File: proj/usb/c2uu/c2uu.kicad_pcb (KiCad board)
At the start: 2 copper layers, 14 x 12 mm, 15 parts, among them J1 USB_C_Receptacle_USB2.0_16P, P1 USB_C_Plug, U1 CH340E, U2 TS5A23159DGS

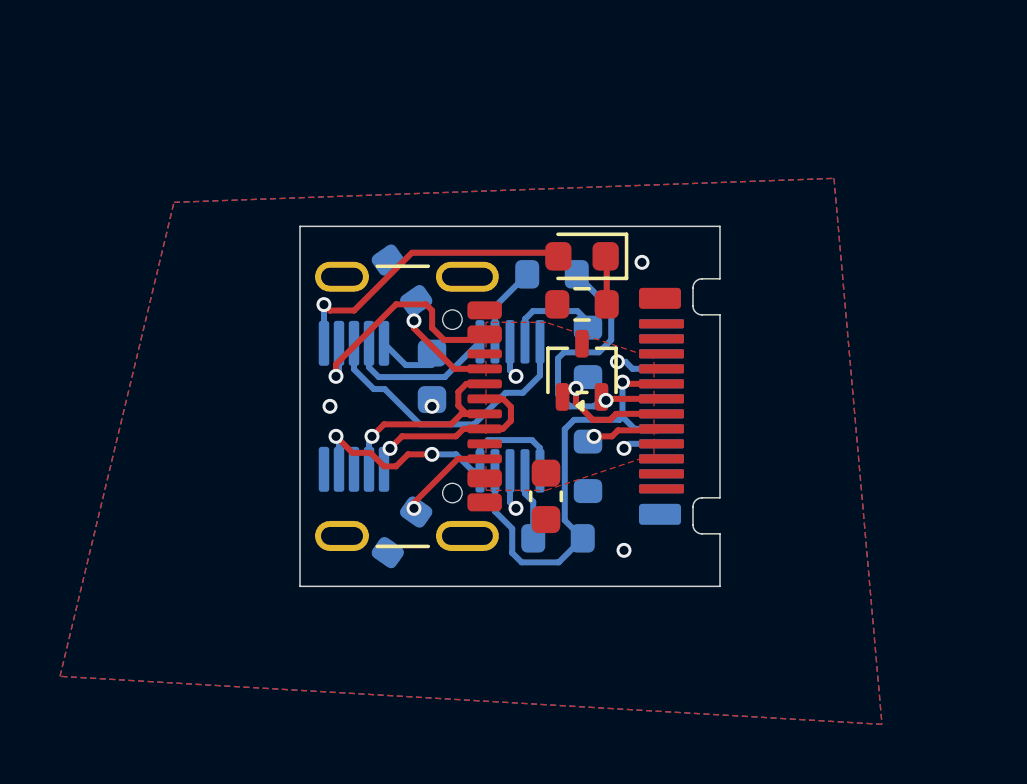
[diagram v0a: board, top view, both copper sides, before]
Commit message: -
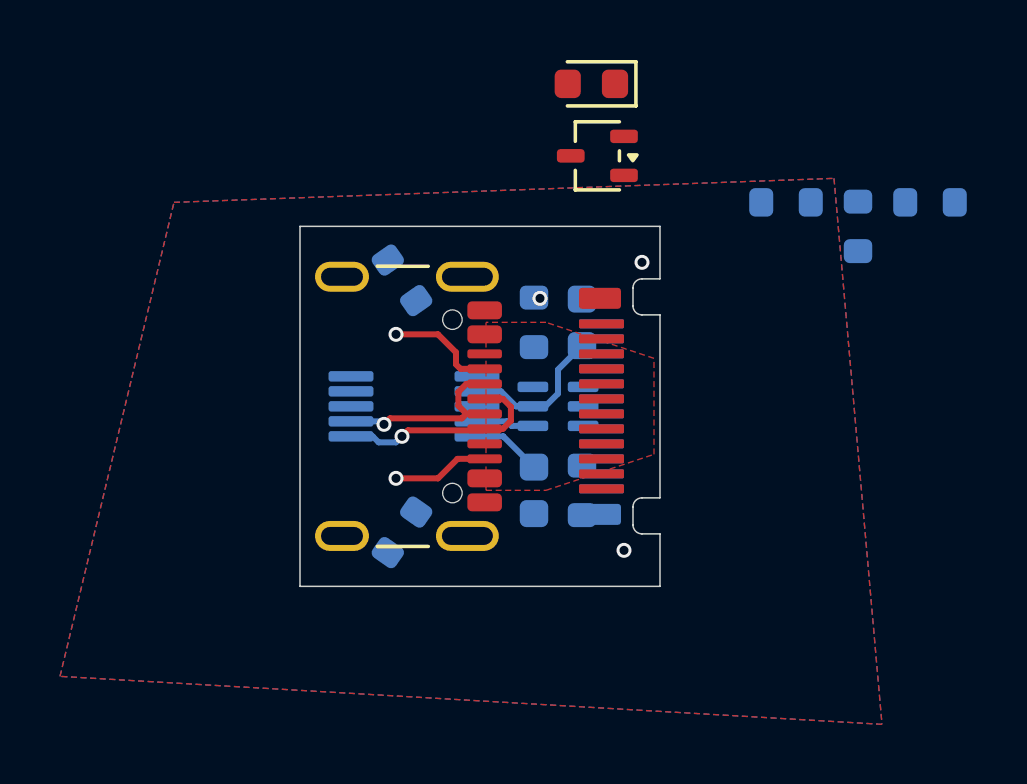
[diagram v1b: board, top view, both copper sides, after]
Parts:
- C1, P1, R7: moved to B.Cu
- U2: value TS5A23159DGS -> 74LVC1G3157; footprint Package_SO:TSSOP-10_3x3mm_P0.5mm -> Package_TO_SOT_SMD:SOT-363_SC-70-6
- moved R5 16.7 mm to (112.0, 93.2)
- moved R4 9.93 mm to (109.6, 94.0)
- moved R6 8.16 mm to (107.2, 93.2)
- moved D2 7.17 mm to (100.9, 91.7), turned to 180 degrees
- moved C1 5.92 mm to (100.4, 97.2), turned to 90 degrees
- moved D1 5.76 mm to (100.7, 89.2)
- moved C2 5.10 mm to (98.8, 102.8)
- moved P1 2.00 mm to (102.1, 100.0), turned to -90 degrees
- moved U1 2.00 mm to (94.8, 100.0), turned to 0 degrees
- moved R7 1.71 mm to (98.8, 97.2), turned to 90 degrees
- moved U2 1.60 mm to (99.6, 100.0), turned to 180 degrees
- moved R3 0.82 mm to (100.4, 102.8)
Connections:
- D1 pad 1: Net-(D1-K) -> GND
- D1 pad 2: TNOW -> Net-(D1-A)
- R4 pad 1: Net-(R4-Pad1) -> TXD
- R5 pad 1: Net-(R5-Pad1) -> TXD
- R7 pad 1: Net-(D1-K) -> TNOW
- R7 pad 2: GND -> Net-(D1-A)
- U2 pad 1: ~{RTS} -> UPDI
- U2 pad 2: Net-(R5-Pad1) -> GND
- U2 pad 3: GND -> Net-(R6-Pad1)
- U2 pad 4: UPDI -> RXD
- U2 pad 5: ~{RTS} -> VBUS
- U2 pad 6: RXD -> ~{RTS}
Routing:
- net UPDI: track 15.5 -> 0.00 mm, vias 1 -> 0
- net ~{RTS}: track 10.5 -> 0.00 mm, vias 2 -> 0
- net TNOW: track 10.0 -> 0.00 mm, vias 1 -> 0
- net UART_IN: track 9.68 -> 0.00 mm, vias 1 -> 0
- net TXD: track 9.63 -> 0.00 mm
- net VBUS: track 12.1 -> 5.01 mm, vias 4 -> 0
- net UART_OUT: track 4.12 -> 0.00 mm, vias 1 -> 0
- net RXD: track 5.12 -> 1.92 mm
- net Net-(R4-Pad1): track 3.11 -> 0.00 mm
- net Net-(R6-Pad1): track 2.70 -> 0.00 mm
- net Net-(R5-Pad1): track 2.36 -> 0.00 mm
- net Net-(P1-CC): track 2.25 -> 0.00 mm, vias 1 -> 0
- net Net-(D1-K): track 1.62 -> 0.00 mm
- net GND: track 1.33 -> 0.00 mm, vias 5 -> 2
- net D-: track 7.64 -> 6.47 mm
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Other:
- board size 14 x 12 mm -> 12 x 12 mm
